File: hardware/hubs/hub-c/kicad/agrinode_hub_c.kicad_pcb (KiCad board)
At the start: 2 copper layers, 130 x 96 mm, 119 parts, among them J1 DC 12V 5.5/2.1, J10 LTE MODULE, J2 DC IN 7-24V, J3 SOLAR 6-24V, J4 USB 5V / PROG, J5 BAT NTC 10k, J6 PROG, J7 I2C, J8 LED STRIP WS2813, J9 RS-485, Q1 AO3401A, Q2 AO3401A, Q3 MMBT3904, Q4 MMBT3904, Q5 BSS138, Q6 MMBT3904, Q7 AO3401A, Q8 MMBT3904, Q9 MMBT3904, SW1 RESET, SW2 BOOT / PAIR, U1 LM2596S-5.0, U2 TP4056, U3 MIC29302WU, U4 ESP32-WROOM-32E-N8, U5 CH340C, U6 DS3231MZ, U7 MAX3485ESA, U8 MIC29302WU

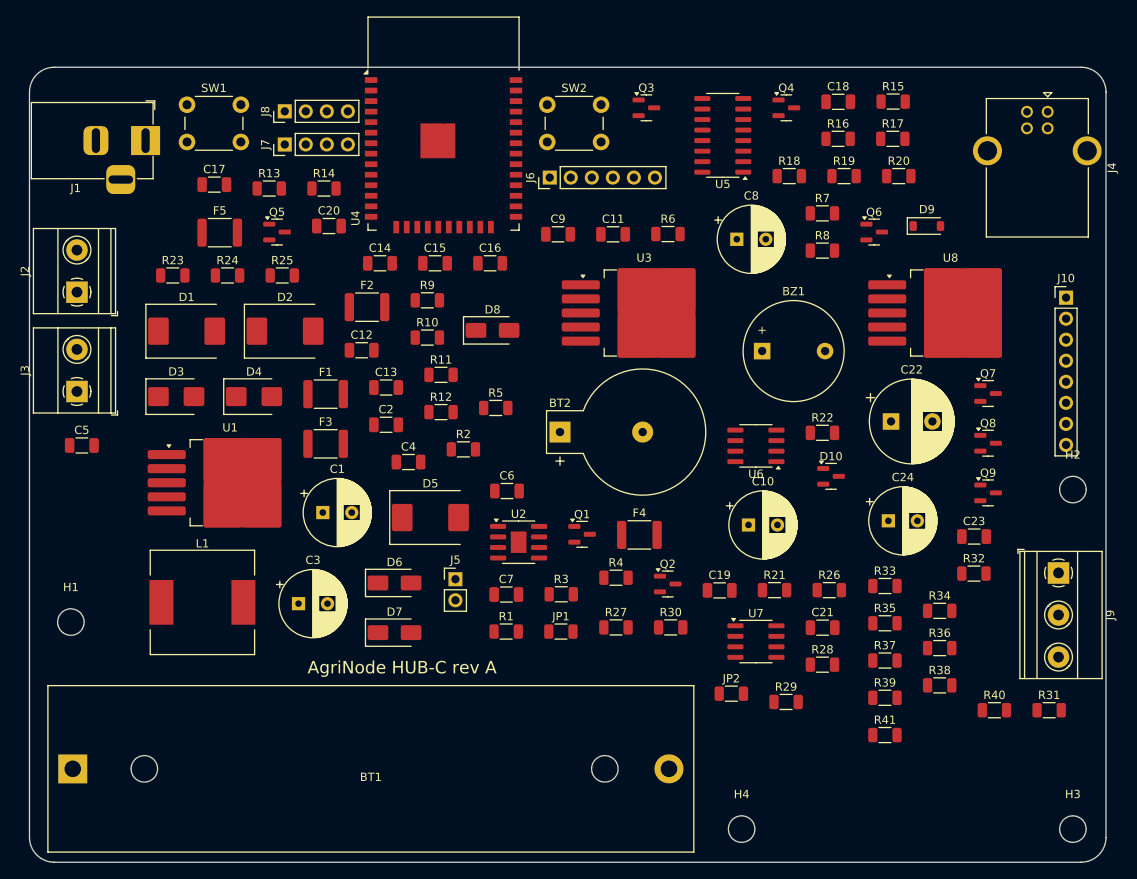
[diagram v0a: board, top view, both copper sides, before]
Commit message: hubs: routing progress snapshot
Co-Authored-By: Claude Opus 5.5 <noreply@anthropic.com>
Claude-Session: https://claude.ai/code/session_014J7amXZ5Y6AZWEh5CjDNja
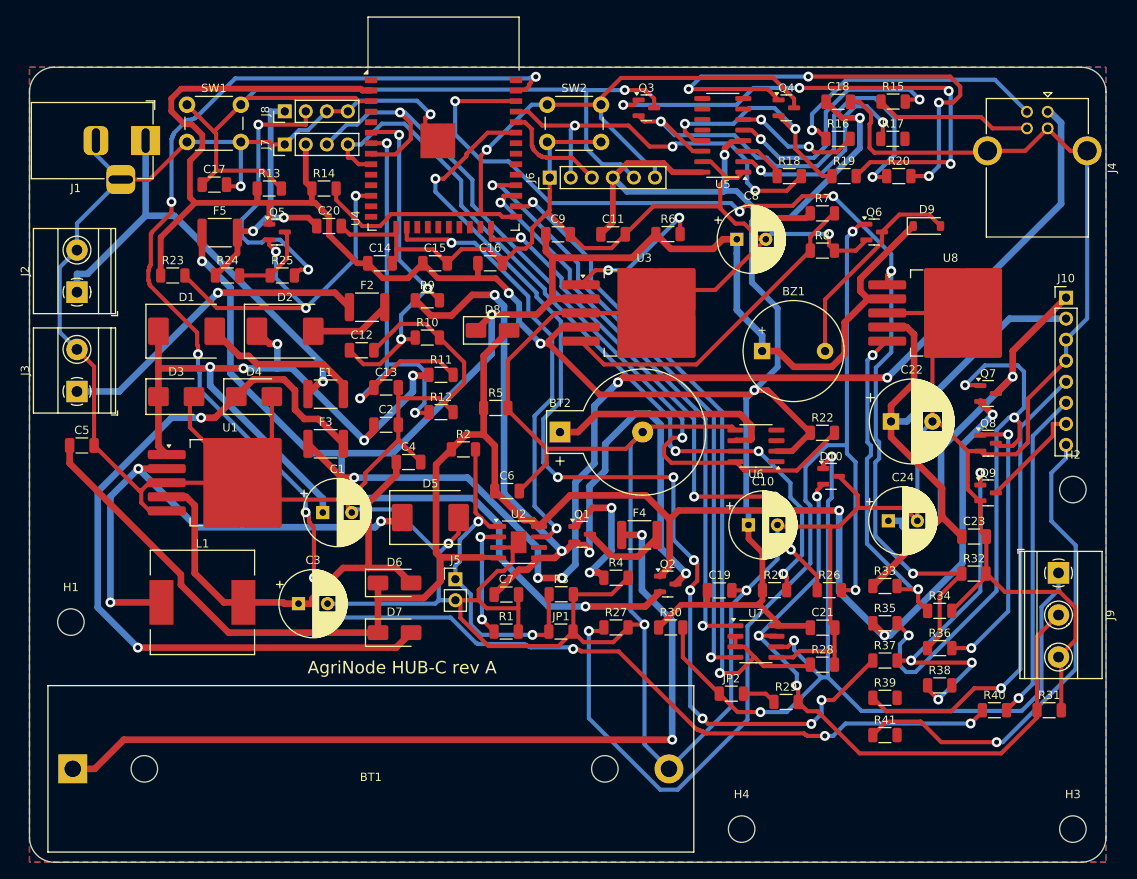
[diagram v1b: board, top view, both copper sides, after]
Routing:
- net GND: track 0.00 -> 839.1 mm, vias 0 -> 6
- net +3V3: track 0.00 -> 316.6 mm, vias 0 -> 6
- net V5: track 0.00 -> 220.8 mm, vias 0 -> 3
- net VSYS: track 0.00 -> 210.3 mm, vias 0 -> 3
- net MODEM_TXD: track 0.00 -> 203.7 mm, vias 0 -> 8
- net /Power - 12V, solar and USB inputs, 18650 charger, rails/VUSB_RAW: track 0.00 -> 140.4 mm, vias 0 -> 5
- net MODEM_EN: track 0.00 -> 131.6 mm, vias 0 -> 5
- net /ESP32, programming, buttons, RTC, LED strip, buzzer/BUZ_B: track 0.00 -> 126.5 mm, vias 0 -> 3
- net MODEM_PWRKEY_CTL: track 0.00 -> 126.4 mm, vias 0 -> 8
- net /ESP32, programming, buttons, RTC, LED strip, buzzer/ESP_EN: track 0.00 -> 107.9 mm, vias 0 -> 1
- net /RS-485 and uplink/RS485_A: track 0.00 -> 106.2 mm, vias 0 -> 3
- net /Power - 12V, solar and USB inputs, 18650 charger, rails/VBAT: track 0.00 -> 104.3 mm, vias 0 -> 4
- net /Power - 12V, solar and USB inputs, 18650 charger, rails/BATT_CELL: track 0.00 -> 102.5 mm, vias 0 -> 2
- net /ESP32, programming, buttons, RTC, LED strip, buzzer/I2C_SCL: track 0.00 -> 100.6 mm, vias 0 -> 2
- net /ESP32, programming, buttons, RTC, LED strip, buzzer/I2C_SDA: track 0.00 -> 95.8 mm, vias 0 -> 3
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- added copper zone on B.Cu, net GND
- added copper zone on F.Cu, net GND

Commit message: hubs: routing progress snapshot
Co-Authored-By: Claude Opus 5.5 <noreply@anthropic.com>
Claude-Session: https://claude.ai/code/session_014J7amXZ5Y6AZWEh5CjDNja
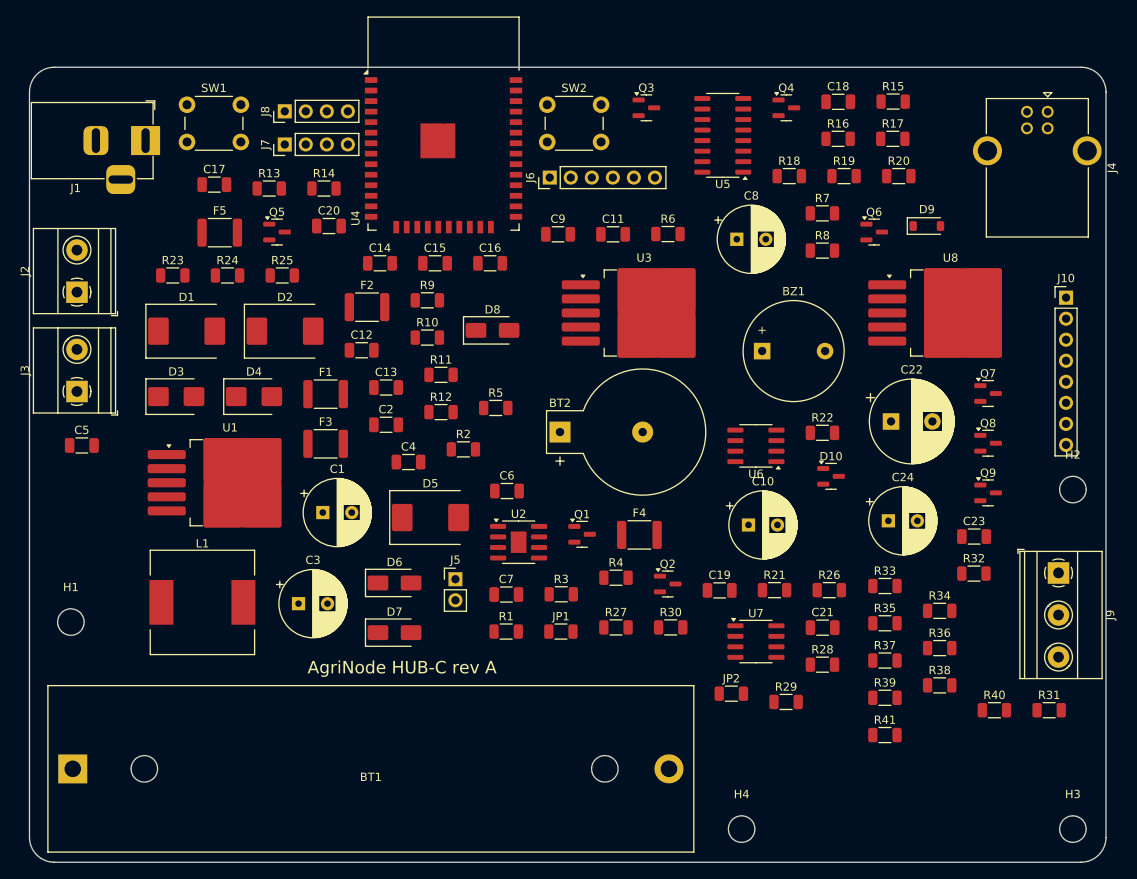
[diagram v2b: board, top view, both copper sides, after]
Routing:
- net GND: track 839.1 -> 0.00 mm, vias 6 -> 0
- net +3V3: track 316.6 -> 0.00 mm, vias 6 -> 0
- net V5: track 220.8 -> 0.00 mm, vias 3 -> 0
- net VSYS: track 210.3 -> 0.00 mm, vias 3 -> 0
- net MODEM_TXD: track 203.7 -> 0.00 mm, vias 8 -> 0
- net /Power - 12V, solar and USB inputs, 18650 charger, rails/VUSB_RAW: track 140.4 -> 0.00 mm, vias 5 -> 0
- net MODEM_EN: track 131.6 -> 0.00 mm, vias 5 -> 0
- net /ESP32, programming, buttons, RTC, LED strip, buzzer/BUZ_B: track 126.5 -> 0.00 mm, vias 3 -> 0
- net MODEM_PWRKEY_CTL: track 126.4 -> 0.00 mm, vias 8 -> 0
- net /ESP32, programming, buttons, RTC, LED strip, buzzer/ESP_EN: track 107.9 -> 0.00 mm, vias 1 -> 0
- net /RS-485 and uplink/RS485_A: track 106.2 -> 0.00 mm, vias 3 -> 0
- net /Power - 12V, solar and USB inputs, 18650 charger, rails/VBAT: track 104.3 -> 0.00 mm, vias 4 -> 0
- net /Power - 12V, solar and USB inputs, 18650 charger, rails/BATT_CELL: track 102.5 -> 0.00 mm, vias 2 -> 0
- net /ESP32, programming, buttons, RTC, LED strip, buzzer/I2C_SCL: track 100.6 -> 0.00 mm, vias 2 -> 0
- net /ESP32, programming, buttons, RTC, LED strip, buzzer/I2C_SDA: track 95.8 -> 0.00 mm, vias 3 -> 0
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- removed copper zone on B.Cu, net GND
- removed copper zone on F.Cu, net GND
